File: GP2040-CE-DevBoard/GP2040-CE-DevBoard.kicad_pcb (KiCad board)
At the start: 2 copper layers, 145 x 61 mm, 51 parts, among them J1 USB_C_Receptacle, J2 Conn_02x22_Odd_Even, J3 Debug, J4 RGB LED, J5 qwiic, SW1 Up, SW10 L2, SW11 B3, SW12 B4, SW13 R1, SW14 L1, SW15 BOOTSEL, SW16 Settings, SW17 A1, SW18 Reset, SW19 A2, SW2 Down, SW3 Left, SW4 Right, SW5 S1, SW6 S2, SW7 B1, SW8 B2, SW9 R2, U1 Raspbery Pi Pico, U2 ADS1219IPWR, U3 ADS1219IPWR, U4 Left Stick, U5 Right Stick

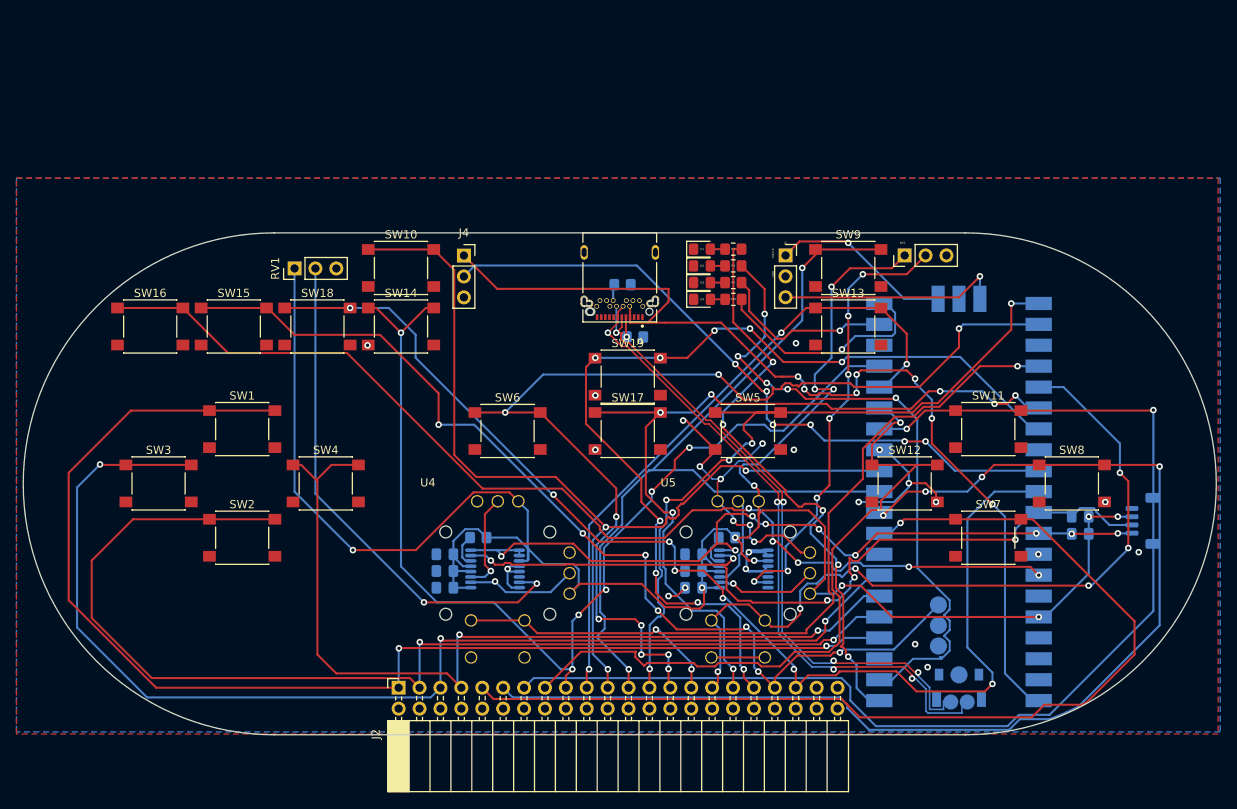
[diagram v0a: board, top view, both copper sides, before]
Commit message: Progress
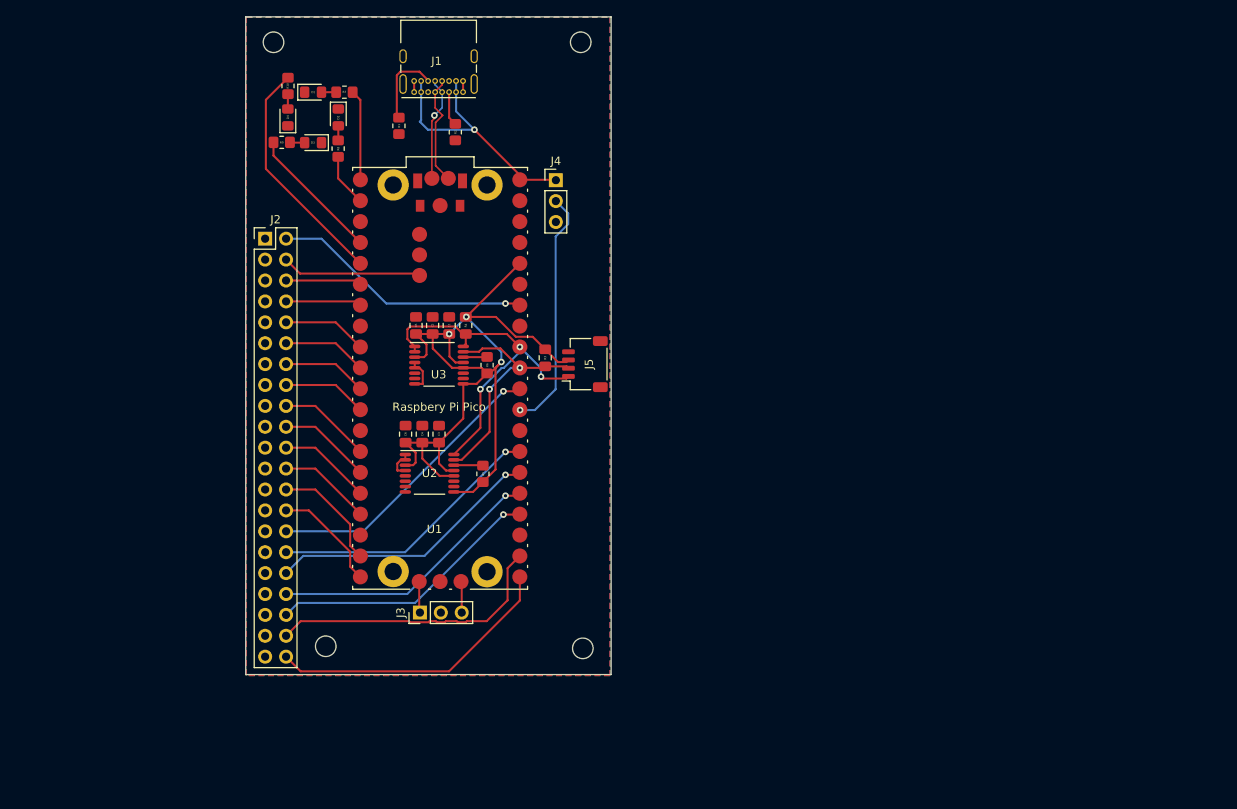
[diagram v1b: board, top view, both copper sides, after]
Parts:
- removed RV1, RV2: 10k, Connector_PinHeader_2.54mm:PinHeader_1x03_P2.54mm_Vertical
- removed SW1: Up, Button_Switch_SMD:SW_Push_1P1T_NO_6x6mm_H9.5mm
- removed SW10: L2, Button_Switch_SMD:SW_Push_1P1T_NO_6x6mm_H9.5mm
- removed SW11: B3, Button_Switch_SMD:SW_Push_1P1T_NO_6x6mm_H9.5mm
- removed SW12: B4, Button_Switch_SMD:SW_Push_1P1T_NO_6x6mm_H9.5mm
- removed SW13: R1, Button_Switch_SMD:SW_Push_1P1T_NO_6x6mm_H9.5mm
- removed SW14: L1, Button_Switch_SMD:SW_Push_1P1T_NO_6x6mm_H9.5mm
- removed SW15: BOOTSEL, Button_Switch_SMD:SW_Push_1P1T_NO_6x6mm_H9.5mm
- removed SW16: Settings, Button_Switch_SMD:SW_Push_1P1T_NO_6x6mm_H9.5mm
- removed SW17: A1, Button_Switch_SMD:SW_Push_1P1T_NO_6x6mm_H9.5mm
- removed SW18: Reset, Button_Switch_SMD:SW_Push_1P1T_NO_6x6mm_H9.5mm
- removed SW19: A2, Button_Switch_SMD:SW_Push_1P1T_NO_6x6mm_H9.5mm
- removed SW2: Down, Button_Switch_SMD:SW_Push_1P1T_NO_6x6mm_H9.5mm
- removed SW3: Left, Button_Switch_SMD:SW_Push_1P1T_NO_6x6mm_H9.5mm
- removed SW4: Right, Button_Switch_SMD:SW_Push_1P1T_NO_6x6mm_H9.5mm
- removed SW5: S1, Button_Switch_SMD:SW_Push_1P1T_NO_6x6mm_H9.5mm
- removed SW6: S2, Button_Switch_SMD:SW_Push_1P1T_NO_6x6mm_H9.5mm
- removed SW7: B1, Button_Switch_SMD:SW_Push_1P1T_NO_6x6mm_H9.5mm
- removed SW8: B2, Button_Switch_SMD:SW_Push_1P1T_NO_6x6mm_H9.5mm
- removed SW9: R2, Button_Switch_SMD:SW_Push_1P1T_NO_6x6mm_H9.5mm
- removed U4: Left Stick, THB001P:THB001P
- removed U5: Right Stick, THB001P:THB001P
- added REF**: MountingHole_2.5mm, MountingHole:MountingHole_2.5mm, F.Cu at (143.5, 126.5)
- added REF**: MountingHole_2.5mm, MountingHole:MountingHole_2.5mm, F.Cu at (105.9, 52.8)
- added REF**: MountingHole_2.5mm, MountingHole:MountingHole_2.5mm, F.Cu at (112.3, 126.2)
- added REF**: MountingHole_2.5mm, MountingHole:MountingHole_2.5mm, F.Cu at (143.3, 52.8)
- C1, C2, C3, C4, C5, C6, R3, R4: footprint ul_NCP1117DT33T5G:C_0805_2012Metric_Pad1.18x1.45mm_HandSolder -> OpenStick:C_0805_2012Metric_Pad1.18x1.45mm_HandSolder; moved to F.Cu
- D1, D2, D3, D4: footprint ul_ADS1219IPWR:LED_0805_2012Metric_Pad1.15x1.40mm_HandSolder -> OpenStick:LED_0805_2012Metric_Pad1.15x1.40mm_HandSolder
- J1: footprint UJ31-CH-31-SMT-TR:CUI_UJ31-CH-31-SMT-TR -> Connector_USB:USB_C_Receptacle_GCT_USB4085
- J2: value Conn_02x22_Odd_Even -> Conn_02x21_Odd_Even; footprint Connector_PinSocket_2.54mm:PinSocket_2x22_P2.54mm_Horizontal -> Connector_PinHeader_2.54mm:PinHeader_2x21_P2.54mm_Vertical
- J3, J4: footprint Connector_PinSocket_2.54mm:PinSocket_1x03_P2.54mm_Vertical -> Connector_PinHeader_2.54mm:PinHeader_1x03_P2.54mm_Vertical
- J5: footprint Connector_JST:JST_SH_BM04B-SRSS-TB_1x04-1MP_P1.00mm_Vertical -> Connector_JST:JST_SH_SM04B-SRSS-TB_1x04-1MP_P1.00mm_Horizontal; moved to F.Cu
- R1, R2, R5, R6: footprint ul_ADS1219IPWR:R_0805_2012Metric_Pad1.20x1.40mm_HandSolder -> OpenStick:R_0805_2012Metric_Pad1.20x1.40mm_HandSolder; moved to F.Cu
- R10, R7, R8, R9: footprint ul_ADS1219IPWR:R_0805_2012Metric_Pad1.20x1.40mm_HandSolder -> OpenStick:R_0805_2012Metric_Pad1.20x1.40mm_HandSolder
- U1: footprint ul_SC0915:SC0915 -> OpenStick:Raspberry Pi Pico - pogo pin and screw mount; moved to F.Cu
- U2, U3: footprint ul_ADS1219IPWR:ADS1219IPWR -> OpenStick:ADS1219IPWR; moved to F.Cu
- moved R4 78.9 mm to (129.3, 87.3), turned to 90 degrees
- moved J5 70.4 mm to (143.8, 91.9)
- moved R3 67.8 mm to (138.9, 91.2), turned to 90 degrees
- moved J3 62.1 mm to (123.7, 122.1), turned to 90 degrees
- moved R10 60.0 mm to (107.7, 58.1), turned to 90 degrees
- moved R9 57.5 mm to (106.9, 65.0), turned to 180 degrees
- moved J2 56.9 mm to (104.9, 76.7), turned to 0 degrees
- moved D4 55.0 mm to (107.7, 62.0), turned to 90 degrees
- moved U1 53.6 mm to (136.7, 119.2)
- moved D1 51.0 mm to (110.7, 58.9)
- moved R7 51.0 mm to (114.5, 58.9)
- moved D3 50.2 mm to (110.7, 65.0), turned to 180 degrees
- moved R8 50.1 mm to (113.8, 65.8), turned to -90 degrees
- moved D2 47.7 mm to (113.8, 62.0), turned to -90 degrees
- moved C5 45.0 mm to (123.2, 87.3), turned to 90 degrees
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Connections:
- J2 pad 1: Up -> GND
- J2 pad 10: GND -> Right
- J2 pad 11: B2 -> GND
- J2 pad 12: GND -> Left
- J2 pad 13: B3 -> GND
- J2 pad 14: GND -> B1
- J2 pad 15: B4 -> GND
- J2 pad 16: GND -> B2
- J2 pad 17: L1 -> GND
- J2 pad 18: GND -> R2
- J2 pad 19: R1 -> GND
- J2 pad 2: GND -> SETTINGS
- J2 pad 20: GND -> L2
- J2 pad 21: L2 -> GND
- J2 pad 22: GND -> B3
- J2 pad 23: R2 -> GND
- J2 pad 24: GND -> B4
- J2 pad 25: S1 -> GND
- J2 pad 26: GND -> R1
- J2 pad 27: S2 -> GND
- J2 pad 28: GND -> L1
- J2 pad 29: L3 -> GND
- J2 pad 3: Down -> GND
- J2 pad 30: GND -> RUN
- J2 pad 31: R3 -> GND
- J2 pad 32: GND -> A2
- J2 pad 33: A1 -> GND
- J2 pad 34: GND -> A1
- J2 pad 35: A2 -> GND
- J2 pad 36: GND -> R3
- J2 pad 37: BOOTSEL -> GND
- J2 pad 38: GND -> L3
- J2 pad 39: RUN -> GND
- J2 pad 4: GND -> BOOTSEL
- J2 pad 40: GND -> S2
- J2 pad 41: (no net) -> GND
- J2 pad 42: (no net) -> S1
- J2 pad 5: Left -> GND
- J2 pad 6: GND -> Up
- J2 pad 7: Right -> GND
- J2 pad 8: GND -> Down
- J2 pad 9: B1 -> GND
- U1 pad 10: B2 -> Left
- U1 pad 11: R2 -> B1
- U1 pad 12: L2 -> B2
- U1 pad 14: B3 -> R2
- U1 pad 15: B4 -> L2
- U1 pad 16: R1 -> B3
- U1 pad 17: L1 -> B4
- U1 pad 19: PLED3 -> R1
- U1 pad 20: PLED4 -> L1
- U1 pad 4: Up -> PLED3
- U1 pad 5: Down -> PLED4
- U1 pad 6: Right -> Up
- U1 pad 7: Left -> Down
- U1 pad 9: B1 -> Right
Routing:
- net +3V3: track 269.7 -> 110.6 mm, vias 12 -> 3
- net Up: track 151.9 -> 9.22 mm, vias 2 -> 0
- net B3: track 144.8 -> 11.4 mm, vias 2 -> 0
- net Left: track 143.7 -> 10.3 mm, vias 3 -> 0
- net B2: track 142.6 -> 10.3 mm, vias 4 -> 0
- net Down: track 137.6 -> 9.22 mm, vias 2 -> 0
- net L1: track 128.6 -> 13.4 mm, vias 6 -> 0
- net B1: track 124.8 -> 10.3 mm, vias 1 -> 0
- net RUN: track 144.2 -> 35.6 mm, vias 7 -> 1
- net BOOTSEL: track 121.5 -> 17.0 mm, vias 7 -> 0
- net L2: track 114.7 -> 11.4 mm, vias 3 -> 0
- net Right: track 109.8 -> 10.3 mm, vias 2 -> 0
- net SETTINGS: track 131.3 -> 31.8 mm, vias 5 -> 1
- net S2: track 129.1 -> 35.1 mm, vias 9 -> 0
- net R2: track 103.6 -> 11.4 mm, vias 2 -> 0
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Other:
- board size 145 x 61 mm -> 44.4 x 79.9 mm
- board text removed: "GND"
- board text removed: "SWCLK"
